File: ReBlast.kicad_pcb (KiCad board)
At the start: 2 copper layers, 50.7 x 64.9 mm, 22 parts, among them J1 MOS_8580_Socket, U1 74HC20, U2 74HC139, U3 ZN428E-8, U4 TLC272, U5 MOS_8580

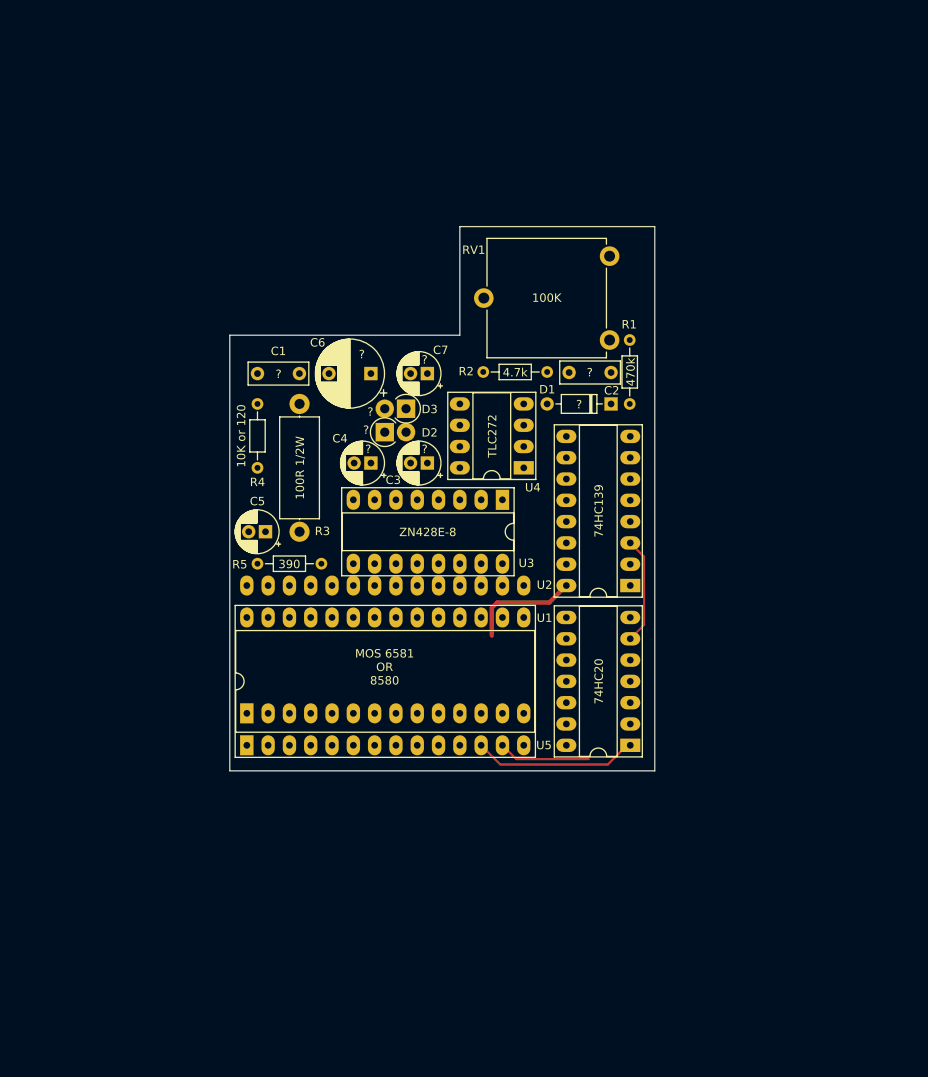
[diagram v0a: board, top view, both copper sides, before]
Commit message: Back side is 99% done. Top side is full of doubts...
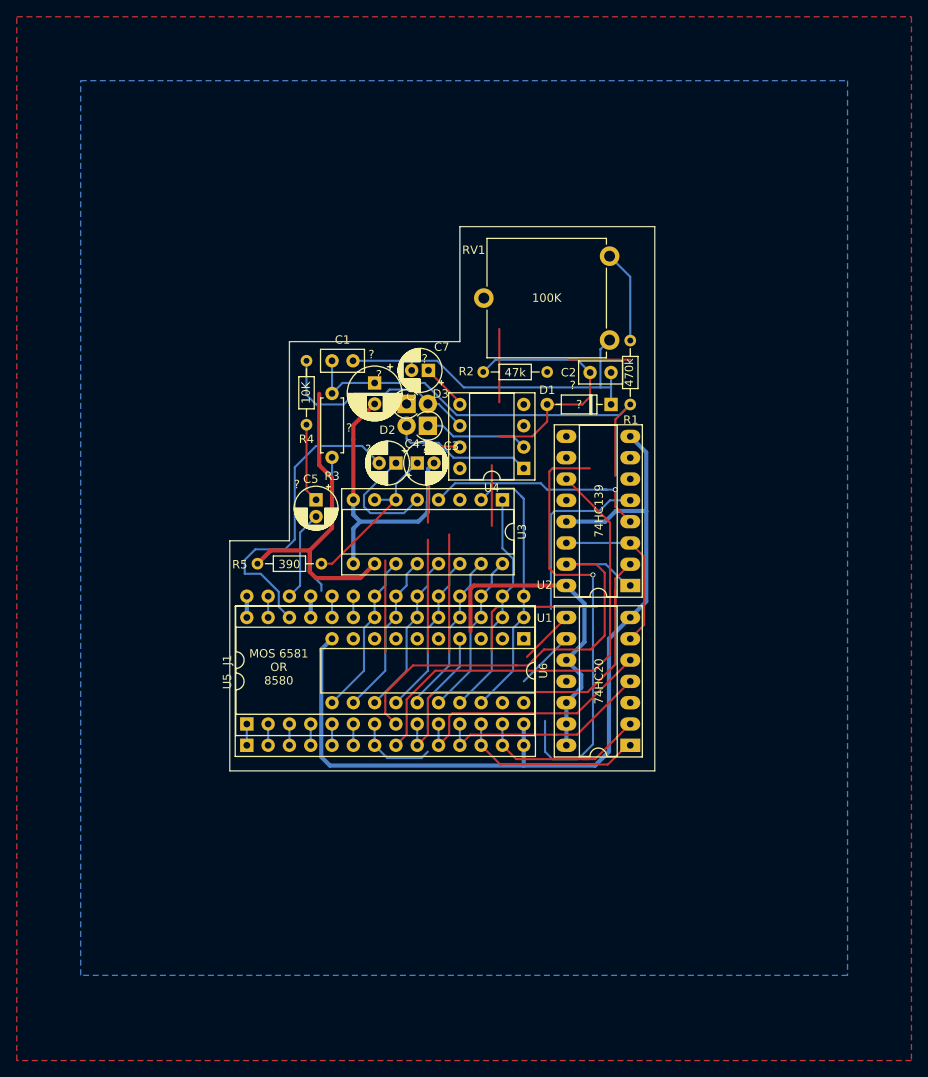
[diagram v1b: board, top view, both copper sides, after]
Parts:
- added U6: ADC0804, Package_DIP:DIP-20_W7.62mm, F.Cu at (162.1, 112.3)
- C1: footprint Capacitor_THT:C_Disc_D7.0mm_W2.5mm_P5.00mm -> Capacitor_THT:C_Disc_D5.0mm_W2.5mm_P2.50mm
- C2: value C_TANTALUM -> 4.7u; footprint Capacitor_THT:C_Disc_D7.0mm_W2.5mm_P5.00mm -> Capacitor_THT:C_Disc_D5.0mm_W2.5mm_P2.50mm
- C4: value CP1 -> C
- C6: footprint Capacitor_THT:CP_Radial_D8.0mm_P5.00mm -> Capacitor_THT:CP_Radial_D6.3mm_P2.50mm
- C7: value CP1 -> 6.8u
- D1: value 1n4148 -> 2.5V ZENER
- J1: footprint ReBlast:DIP-28_Socket_LongPads -> Package_DIP:DIP-28_W15.24mm
- R2: value 4.7k -> 47k
- R3: footprint Resistor_THT:R_Axial_DIN0414_L11.9mm_D4.5mm_P15.24mm_Horizontal -> Resistor_THT:R_Axial_DIN0207_L6.3mm_D2.5mm_P7.62mm_Horizontal
- R4: value 10K or 120 -> 10K
- U3: footprint Package_DIP:DIP-16_W7.62mm_Socket_LongPads -> Package_DIP:DIP-16_W7.62mm_Socket
- U4: footprint Package_DIP:DIP-8_W7.62mm_Socket_LongPads -> Package_DIP:DIP-8_W7.62mm_Socket
- U5: footprint Package_DIP:DIP-28_W15.24mm_Socket_LongPads -> Package_DIP:DIP-28_W15.24mm_Socket
- moved R4 7.78 mm to (136.1, 79.1)
- moved R1 7.68 mm to (174.8, 84.3), turned to 90 degrees
- moved C5 7.13 mm to (137.3, 95.7), turned to 270 degrees
- moved D2 5.20 mm to (150.6, 86.9), turned to 180 degrees
- moved C2 5.00 mm to (172.5, 80.5), turned to 180 degrees
- moved C1 4.18 mm to (139.2, 79.1), turned to 0 degrees
- moved R3 4.07 mm to (139.2, 83.0)
- moved C4 2.98 mm to (146.8, 91.3)
- moved J1 1.27 mm to (129.0, 122.4)
- moved C3 1.21 mm to (149.4, 91.3), turned to 0 degrees
- moved C6 1.20 mm to (144.3, 81.8), turned to 270 degrees
- moved D3 0.58 mm to (148.1, 84.3), turned to 0 degrees
- moved C7 0.40 mm to (150.7, 80.3)
- moved D1 0.06 mm to (172.5, 84.3)
- moved U4 0.06 mm to (162.1, 91.9)
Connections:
- net /~cs_adc_r renamed Net-(U2-Pad9)
- net /~cs_adc_w renamed Net-(U2-Pad10)
- net /~cs_dac_w renamed Net-(U2-Pad12)
- net Net-(C3-Pad1) renamed /vref
- C2 pad 1: Net-(C2-Pad1) -> Net-(C1-Pad2)
- C4 pad 1: Net-(C4-Pad1) -> /dac_output
- C4 pad 2: Net-(C4-Pad2) -> /audio_in
- C5 pad 2: Net-(C5-Pad2) -> /audio_jack
- C6 pad 1: Net-(C6-Pad1) -> Net-(C1-Pad1)
- C6 pad 2: Net-(C6-Pad2) -> GNDA
- C7 pad 2: Net-(C7-Pad2) -> Net-(C1-Pad2)
- D1 pad 1: Net-(D1-Pad1) -> Net-(C1-Pad2)
- D1 pad 2: Net-(D1-Pad2) -> Net-(C2-Pad2)
- D3 pad 1: GNDD -> Net-(C5-Pad1)
- D3 pad 2: Net-(D2-Pad1) -> Net-(D3-Pad2)
- J1 pad 14: GNDD -> GNDA
- J1 pad 26: Net-(J1-Pad26) -> /audio_jack
- R1 pad 1: Net-(R1-Pad1) -> Net-(C1-Pad1)
- R2 pad 2: Net-(R2-Pad2) -> Net-(C2-Pad2)
- R3 pad 1: Net-(R3-Pad1) -> Net-(C1-Pad1)
- R4 pad 1: Net-(R4-Pad1) -> Net-(D3-Pad2)
- R4 pad 2: Net-(R4-Pad2) -> Net-(C5-Pad1)
- RV1 pad 1: Net-(RV1-Pad1) -> Net-(R1-Pad2)
- RV1 pad 3: Net-(RV1-Pad3) -> Net-(C1-Pad2)
- U1 pad 10: Net-(U1-Pad10) -> +5V
- U1 pad 12: Net-(U1-Pad12) -> +5V
- U1 pad 13: Net-(U1-Pad13) -> +5V
- U1 pad 2: /a2 -> /a4
- U1 pad 4: /a1 -> /a2
- U1 pad 5: /a4 -> /a1
- U1 pad 7: GNDD -> GNDA
- U2 pad 11: /~cs_dac_r -> /~cs_sid
- U2 pad 13: /a0 -> GNDA
- U2 pad 14: /r_~w -> /~digiaddr
- U2 pad 15: /~cs_dac_adc -> /~cs_in
- U2 pad 2: GNDD -> /a0
- U2 pad 4: /~cs_dac_adc -> /~cs_dac
- U2 pad 5: Net-(U2-Pad5) -> /~cs_adc
- U2 pad 6: /~cs_sid -> Net-(U2-Pad6)
- U2 pad 8: GNDD -> GNDA
- U3 pad 1: /d6 -> /d1
- U3 pad 11: /d0 -> /d7
- U3 pad 12: /d1 -> /d6
- U3 pad 13: /d2 -> /d5
- U3 pad 14: /d3 -> /d4
- U3 pad 15: /d4 -> /d3
- U3 pad 16: /d5 -> /d2
- U3 pad 2: /d7 -> /d0
- U3 pad 4: Net-(U3-Pad4) -> /~cs_dac
- U3 pad 5: Net-(U3-Pad5) -> /dac_output
- U3 pad 9: GNDD -> GNDA
- U4 pad 1: Net-(U4-Pad1) -> Net-(D2-Pad2)
- U4 pad 2: Net-(U4-Pad2) -> Net-(D2-Pad1)
- U4 pad 4: Net-(U4-Pad4) -> GNDA
- U4 pad 5: Net-(U4-Pad5) -> Net-(C7-Pad1)
- U4 pad 6: Net-(U4-Pad6) -> Net-(D3-Pad2)
- U4 pad 8: Net-(U4-Pad8) -> +5V
- U5 pad 14: GNDD -> GNDA
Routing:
- net GNDA: track 0.00 -> 140.8 mm
- net (no net): track 0.00 -> 137.4 mm, vias 0 -> 1
- net +5V: track 13.3 -> 80.1 mm
- net /~cs_sid: track 0.00 -> 55.6 mm
- net /~cs_in: track 0.00 -> 54.9 mm
- net Net-(C1-Pad1): track 0.00 -> 51.3 mm
- net /a0: track 0.00 -> 47.5 mm
- net Net-(C1-Pad2): track 0.00 -> 43.1 mm
- net /audio_in: track 0.00 -> 37.7 mm
- net /d0: track 0.00 -> 32.9 mm
- net Net-(C2-Pad2): track 0.00 -> 30.9 mm
- net /a1: track 0.00 -> 30.9 mm
- net /d1: track 0.00 -> 27.3 mm
- net /~cs_dac: track 0.00 -> 27.3 mm, vias 0 -> 1
- net /a2: track 0.00 -> 26.0 mm
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- added copper zone on B.Cu, net GNDD
- added copper zone on F.Cu, net GNDD
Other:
- outline, holes or cut-outs redrawn

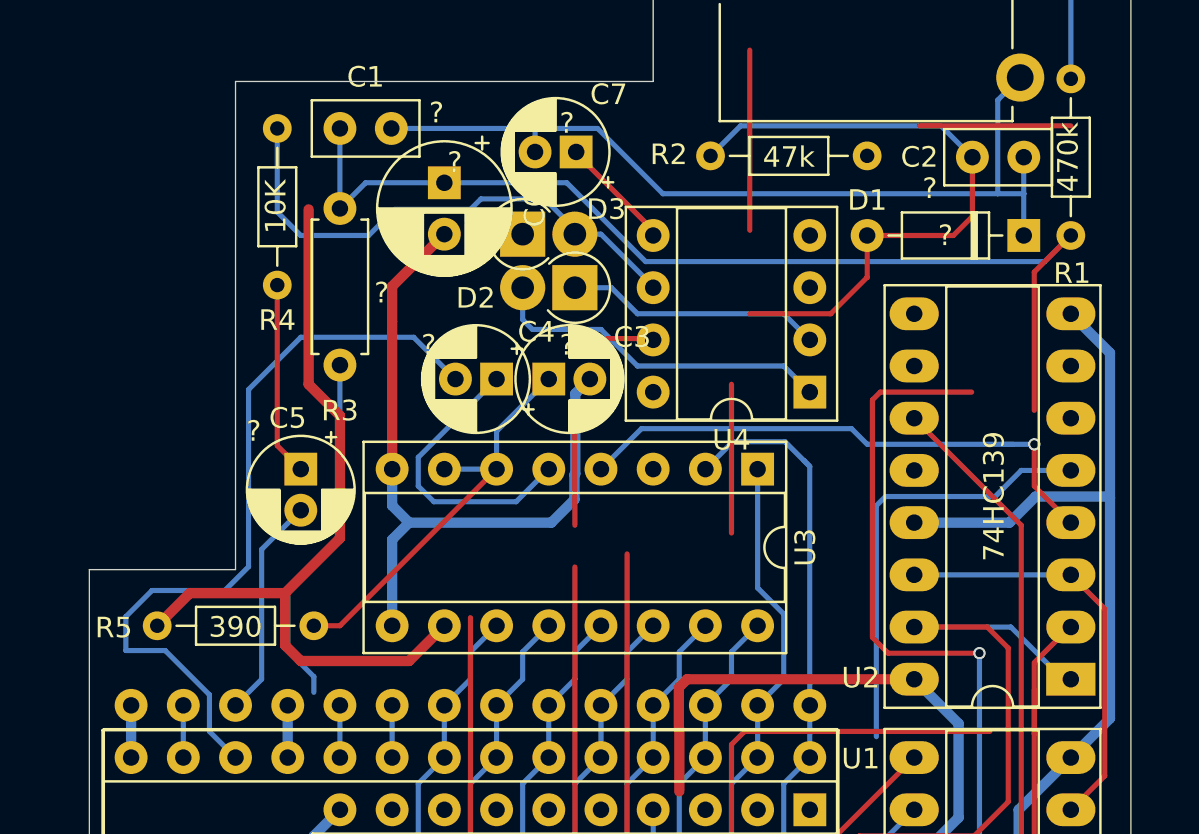
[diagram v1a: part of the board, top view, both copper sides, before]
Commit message: Power circuit almost makes sense
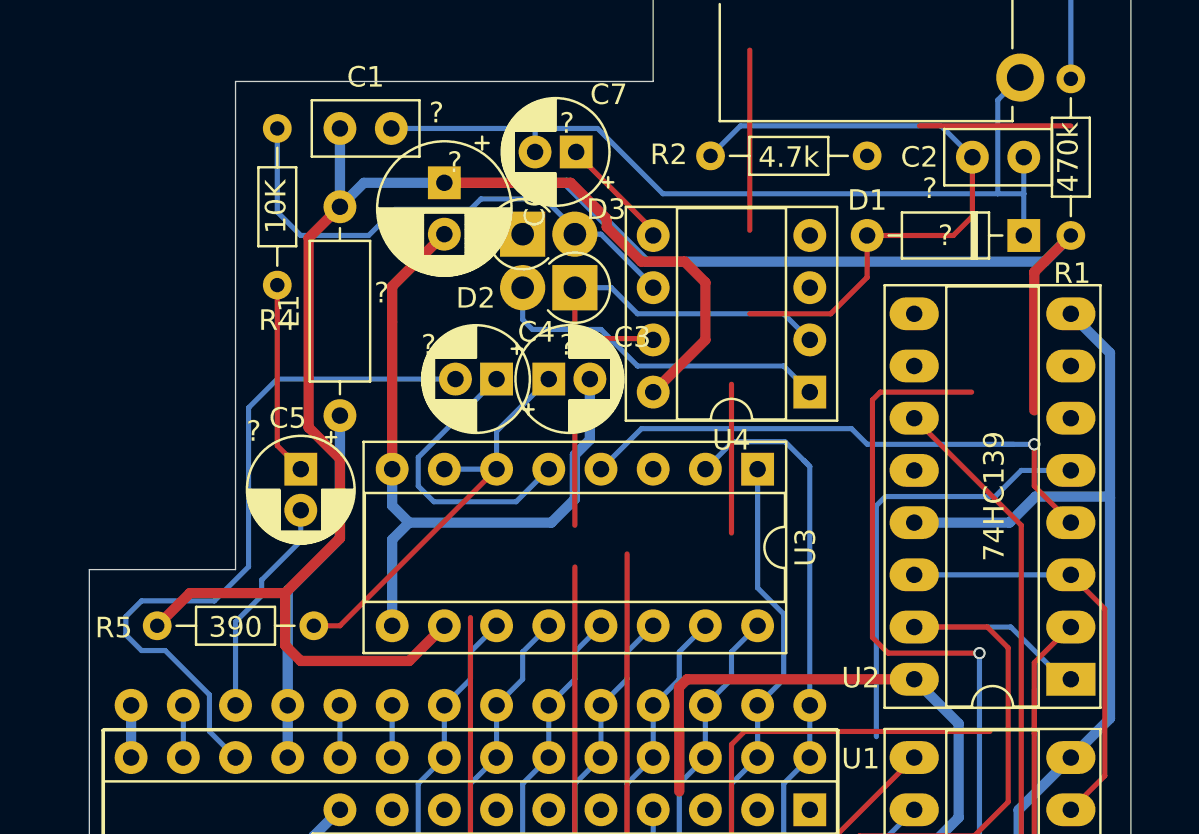
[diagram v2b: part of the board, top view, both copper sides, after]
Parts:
- removed R3: 100R 1/2W, Resistor_THT:R_Axial_DIN0207_L6.3mm_D2.5mm_P7.62mm_Horizontal
- added L1: 100, Inductor_THT:L_Axial_L6.6mm_D2.7mm_P10.16mm_Horizontal_Vishay_IM-2, F.Cu at (139.2, 93.1)
- R2: value 47k -> 4.7k
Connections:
- C1 pad 1: Net-(C1-Pad1) -> +5V
- C6 pad 1: Net-(C1-Pad1) -> +5V
- D3 pad 1: Net-(C5-Pad1) -> Net-(D3-Pad1)
- J1 pad 25: +5V -> VCC
- R1 pad 1: Net-(C1-Pad1) -> +5V
- U5 pad 25: +5V -> VCC
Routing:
- net +5V: track 80.1 -> 150.9 mm
- net Net-(C1-Pad1): track 51.3 -> 0.00 mm
- net VCC: track 0.00 -> 17.7 mm
- net Net-(R3-Pad2): track 17.5 -> 0.00 mm
- net /audio_in: track 37.7 -> 35.1 mm
- net Net-(D2-Pad1): track 12.5 -> 14.6 mm
- net Net-(U4-Pad7): track 2.22 -> 4.10 mm
